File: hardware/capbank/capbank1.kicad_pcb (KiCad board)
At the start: 2 copper layers, 99 x 70.5 mm, 116 parts, among them J1 Screws, J3 Conn_01x02, J4 Conn_01x02, J5 Conn_01x06, K1 3570.1333.121 COMUS, K2 3570.1333.121 COMUS, K4 3570.1333.121 COMUS, SW2 SW_SPST, U1 ULN2003, U10 TS861IL, U11 NXJ1S1212MC, U12 LM317AEMP, U13 74HC14, U14 MCP1415, U15 MCP1415, U16 LM78L05ACZ, U2 OPA2202IDR, U3 MCP1525-TO, U4 MCP4921-EP, U5 PAI130M61, U6 ATtiny84A-P, U7 4046, U9 LM78L05ACZ, Y1 16MHz

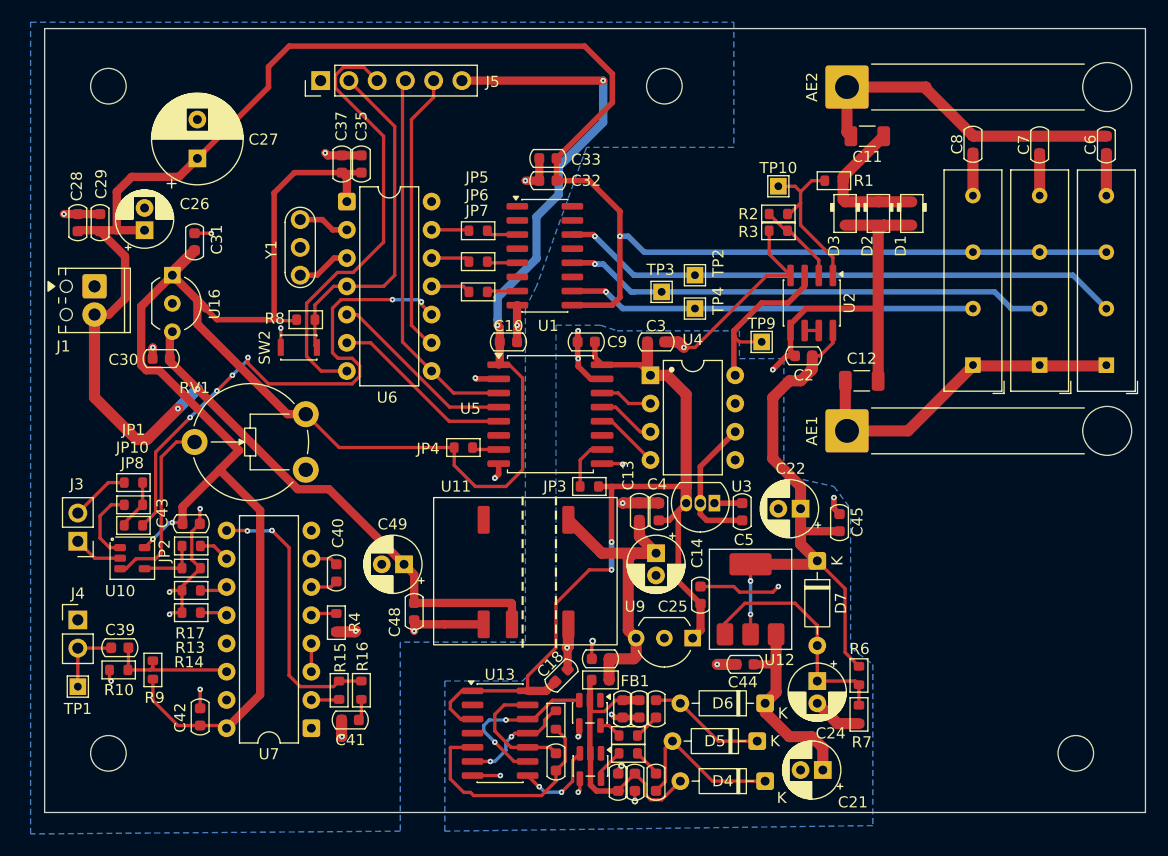
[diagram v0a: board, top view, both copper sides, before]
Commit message: Small hardware changes
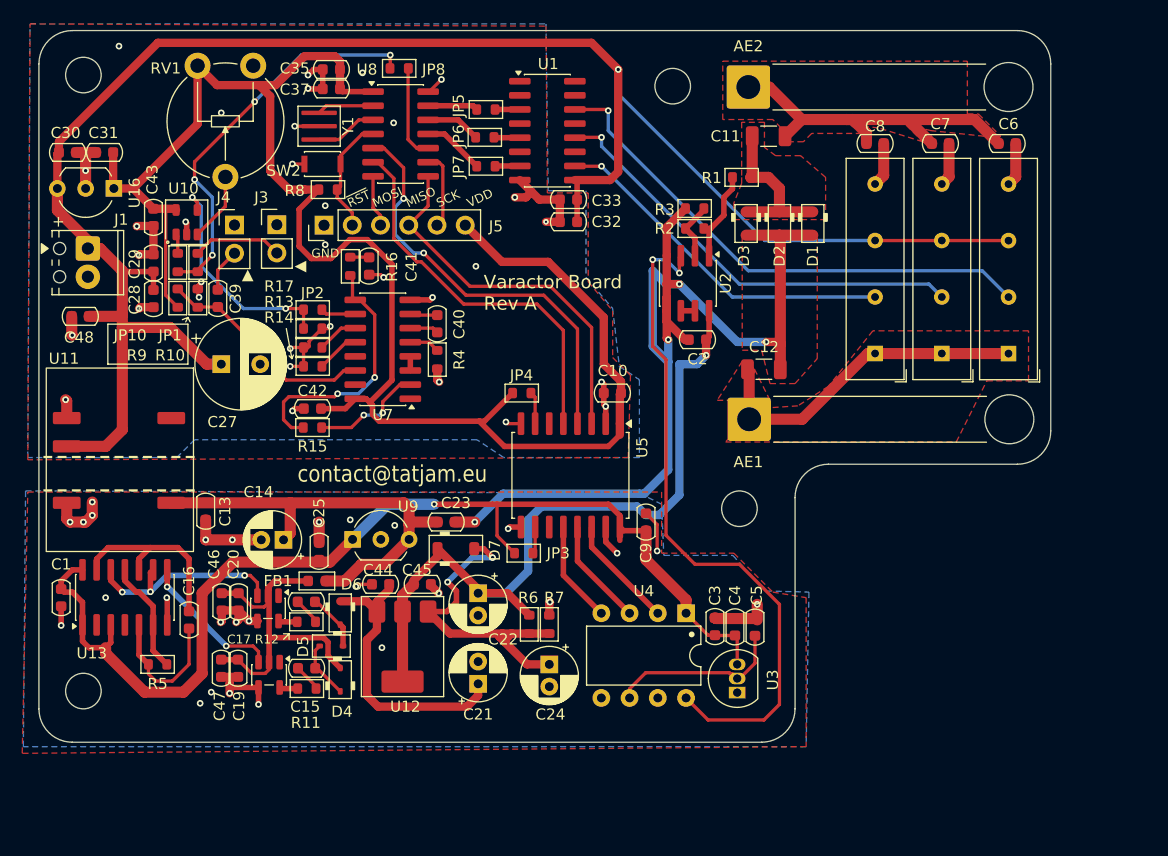
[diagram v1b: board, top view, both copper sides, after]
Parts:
- removed C18: 100n, PCM_Capacitor_SMD_AKL:C_0603_1608Metric
- removed C26, C49: 10u, PCM_Capacitor_THT_AKL:CP_Radial_D5.0mm_P2.00mm
- removed TP1, TP10, TP2, TP3, TP4, TP9: ~, TestPoint:TestPoint_THTPad_1.5x1.5mm_Drill0.7mm
- removed U6: ATtiny84A-P, Package_DIP:DIP-14_W7.62mm
- added C1: 100n, PCM_Capacitor_SMD_AKL:C_0603_1608Metric, F.Cu at (101.0, 100.0)
- added U8: ATtiny84A-SS, Package_SO:SOIC-14_3.9x8.7mm_P1.27mm, F.Cu at (131.5, 58.3)
- D4, D5, D6: value 1N5711 -> BAT46WJ; footprint Diode_THT:D_DO-35_SOD27_P7.62mm_Horizontal -> PCM_Diode_SMD_AKL:D_SOD-323
- D7: value 1N4007 -> 1N4007W; footprint Diode_THT:D_DO-35_SOD27_P7.62mm_Horizontal -> PCM_Diode_SMD_AKL:D_SOD-123
- U7: value 4046 -> 74HC4046AD; footprint Package_DIP:DIP-16_W7.62mm -> Package_SO:SOIC-16_3.9x9.9mm_P1.27mm
- Y1: footprint Crystal:Resonator-3Pin_W7.0mm_H2.5mm -> PCM_Crystal_Handsoldering_AKL:Resonator_SMD_muRata_CSTxExxV-3Pin_3.0x1.1mm_BigPads
- moved JP8 47.5 mm to (131.4, 52.4)
- moved C41 40.9 mm to (128.7, 70.2), turned to -90 degrees
- moved C46 40.5 mm to (115.5, 100.4)
- moved C48 40.1 mm to (102.7, 74.7), turned to 180 degrees
- moved D4 39.3 mm to (126.1, 107.4), turned to 90 degrees
- moved D5 39.2 mm to (125.3, 104.3)
- moved D6 39.1 mm to (126.1, 101.4), turned to -90 degrees
- moved C13 39.0 mm to (114.0, 92.2), turned to -90 degrees
- moved J4 38.2 mm to (116.6, 66.5)
- moved R16 38.1 mm to (127.0, 70.2), turned to 90 degrees
- moved C45 37.9 mm to (133.5, 98.8), turned to 0 degrees
- moved C20 37.8 mm to (117.0, 100.4), turned to -90 degrees
- moved H1 37.4 mm to (162.0, 92.0)
- moved C19 36.3 mm to (116.9, 106.3)
- moved C47 36.3 mm to (115.4, 106.3)
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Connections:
- J1 pad 1: GND -> V_SUPPLY
- J1 pad 2: V_SUPPLY -> GND
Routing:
- net V_SUPPLY: track 213.2 -> 167.4 mm, vias 3 -> 1
- net /Isolated/VTUNE: track 15.8 -> 61.4 mm, vias 0 -> 2
- net VDD: track 201.5 -> 156.9 mm, vias 4 -> 0
- net GND_ISOL: track 100.1 -> 140.6 mm, vias 17 -> 31
- net /Microcontroller/HVSP_CLK_FSK_IN: track 48.4 -> 9.27 mm, vias 6 -> 0
- net /Microcontroller/PRG_MOSI_I2C_SDA: track 39.5 -> 4.67 mm
- net /Microcontroller/FSK_DEMOD: track 4.53 -> 35.9 mm, vias 0 -> 4
- net /SCK: track 17.1 -> 38.2 mm, vias 0 -> 2
- net /Microcontroller/~{RESET}: track 31.4 -> 10.7 mm
- net /SDI: track 16.6 -> 34.9 mm
- net /Microcontroller/PRG_SCK_I2C_SCL: track 25.3 -> 7.00 mm
- net VDD_ISOL: track 84.5 -> 100.0 mm, vias 2 -> 1
- net HV_CLEAN: track 52.6 -> 67.9 mm, vias 2 -> 1
- net /Microcontroller/FSK Demod/FSK_DEMOD: track 5.53 -> 20.4 mm, vias 0 -> 2
- net V_SUPPLY_ISOL: track 28.9 -> 39.7 mm
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- added copper zone on F.Cu, net /Isolated/ANT1
- added copper zone on F.Cu, net /Isolated/ANT2
- added copper zone on F.Cu, net GND
- added copper zone on F.Cu, net GND_ISOL
- added copper zone on F.Cu, net Net-(D1-K)
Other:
- board size 99 x 70.5 mm -> 91 x 64 mm
- board text added: "+"
- board text added: "GND"
- board text added: "MISO"
- board text added: "MOSI"
- board text added: "SCK"
- board text added: "VDD"
- board text added: "Varactor Board Rev A"
- board text added: "contact@tatjam.eu"
- board text added: "~{RST}"
- board text added: "▲"
